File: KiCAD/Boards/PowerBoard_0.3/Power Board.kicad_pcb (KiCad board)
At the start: 2 copper layers, 100 x 162.8 mm, 24 parts, among them J1 Screw_Terminal_01x02, J11 Conn_01x02, J12 Conn_01x09, J13 Conn_01x09, J2 Screw_Terminal_01x02, J3 Conn_01x03, J4 Screw_Terminal_01x02, J5 Conn_01x02, J6 Screw_Terminal_01x02, J7 Screw_Terminal_01x02, J8 Screw_Terminal_01x02, J9 Conn_02x05_Odd_Even, SW1 SW_DPST, SW2 SW_3PDT_x3, SW3 SW_SPST, SW4 SW_SPST, SW5 SW_SPST

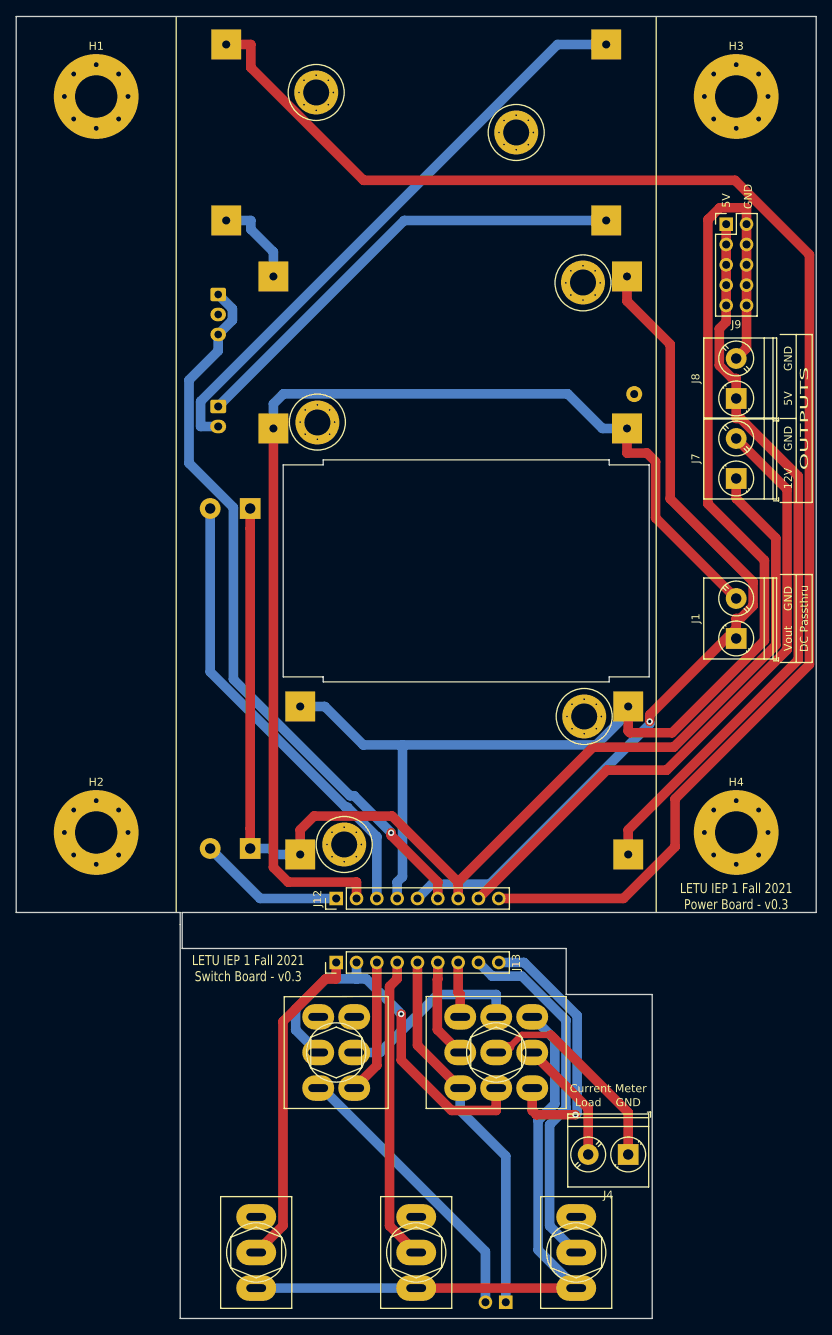
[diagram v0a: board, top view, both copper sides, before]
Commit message: all: More work.
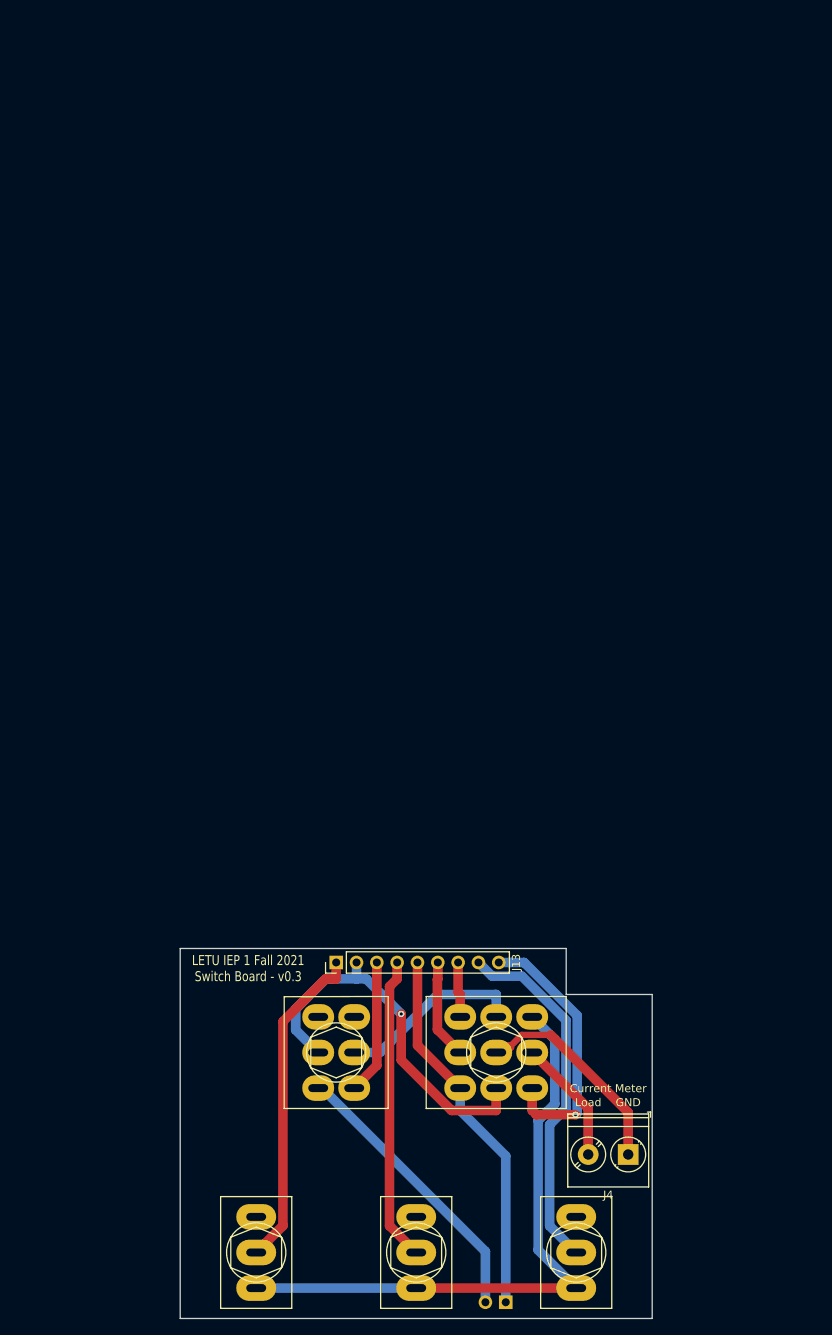
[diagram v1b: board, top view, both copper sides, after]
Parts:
- removed B1: BuckConverter, Custom:BuckConverter
- removed B2: BuckBoostConverter, Custom:BuckBoostConverter
- removed CC1: CurrentLimiter, Custom:ConstantCurrentModule
- removed H1, H2, H3, H4: MountingHole, MountingHole:MountingHole_5.3mm_M5_Pad_Via
- removed J1, J2, J6, J7, J8: Screw_Terminal_01x02, TerminalBlock_Phoenix:TerminalBlock_Phoenix_PT-1,5-2-5.0-H_1x02_P5.00mm_Horizontal
- removed J12: Conn_01x09, Connector_PinHeader_2.54mm:PinHeader_1x09_P2.54mm_Vertical
- removed J3: Conn_01x03, Connector_JST:JST_XH_B3B-XH-A_1x03_P2.50mm_Vertical
- removed J5: Conn_01x02, Connector_JST:JST_XH_B2B-XH-A_1x02_P2.50mm_Vertical
- removed J9: Conn_02x05_Odd_Even, Connector_PinHeader_2.54mm:PinHeader_2x05_P2.54mm_Vertical
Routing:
- net /Switches/CC_-: track 191.2 -> 0.00 mm
- net /Switches/5V_-: track 170.2 -> 0.00 mm
- net +12V: track 153.0 -> 0.00 mm
- net /Switches/DC_-: track 146.0 -> 0.00 mm
- net /Switches/DC_+: track 107.5 -> 0.00 mm, vias 1 -> 0
- net Net-(B1-Pad3): track 92.6 -> 0.00 mm
- net /Switches/Meter_+: track 91.7 -> 0.00 mm, vias 1 -> 0
- net /Switches/12V_-: track 80.5 -> 0.00 mm
- net Net-(CC1-Pad4): track 74.5 -> 0.00 mm
- net Net-(CC1-Pad3): track 58.1 -> 0.00 mm
- net /Switches/BAT_-: track 57.5 -> 0.00 mm
- net /Switches/USB_-: track 18.3 -> 0.00 mm
- net Net-(B2-Pad3): track 11.2 -> 0.00 mm
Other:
- board size 100 x 162.8 mm -> 59 x 46.2 mm
- board text removed: "12V"
- board text removed: "12V+"
- board text removed: "5V"
- board text removed: "Battery Input"
- board text removed: "Charger Output"
- board text removed: "DC Passthru"
- board text removed: "LETU IEP 1 Fall 2021 Power Board - v0.3"
- board text removed: "Meter Power"
- board text removed: "OUTPUTS"
- board text removed: "USB Module"
- board text removed: "V+"
- board text removed: "Vout"
